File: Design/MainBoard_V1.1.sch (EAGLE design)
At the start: 65 parts, among them IC3 LM2936MP-3.3, Q1 25meg, Q4 2N3704, U1 STM32F20XR

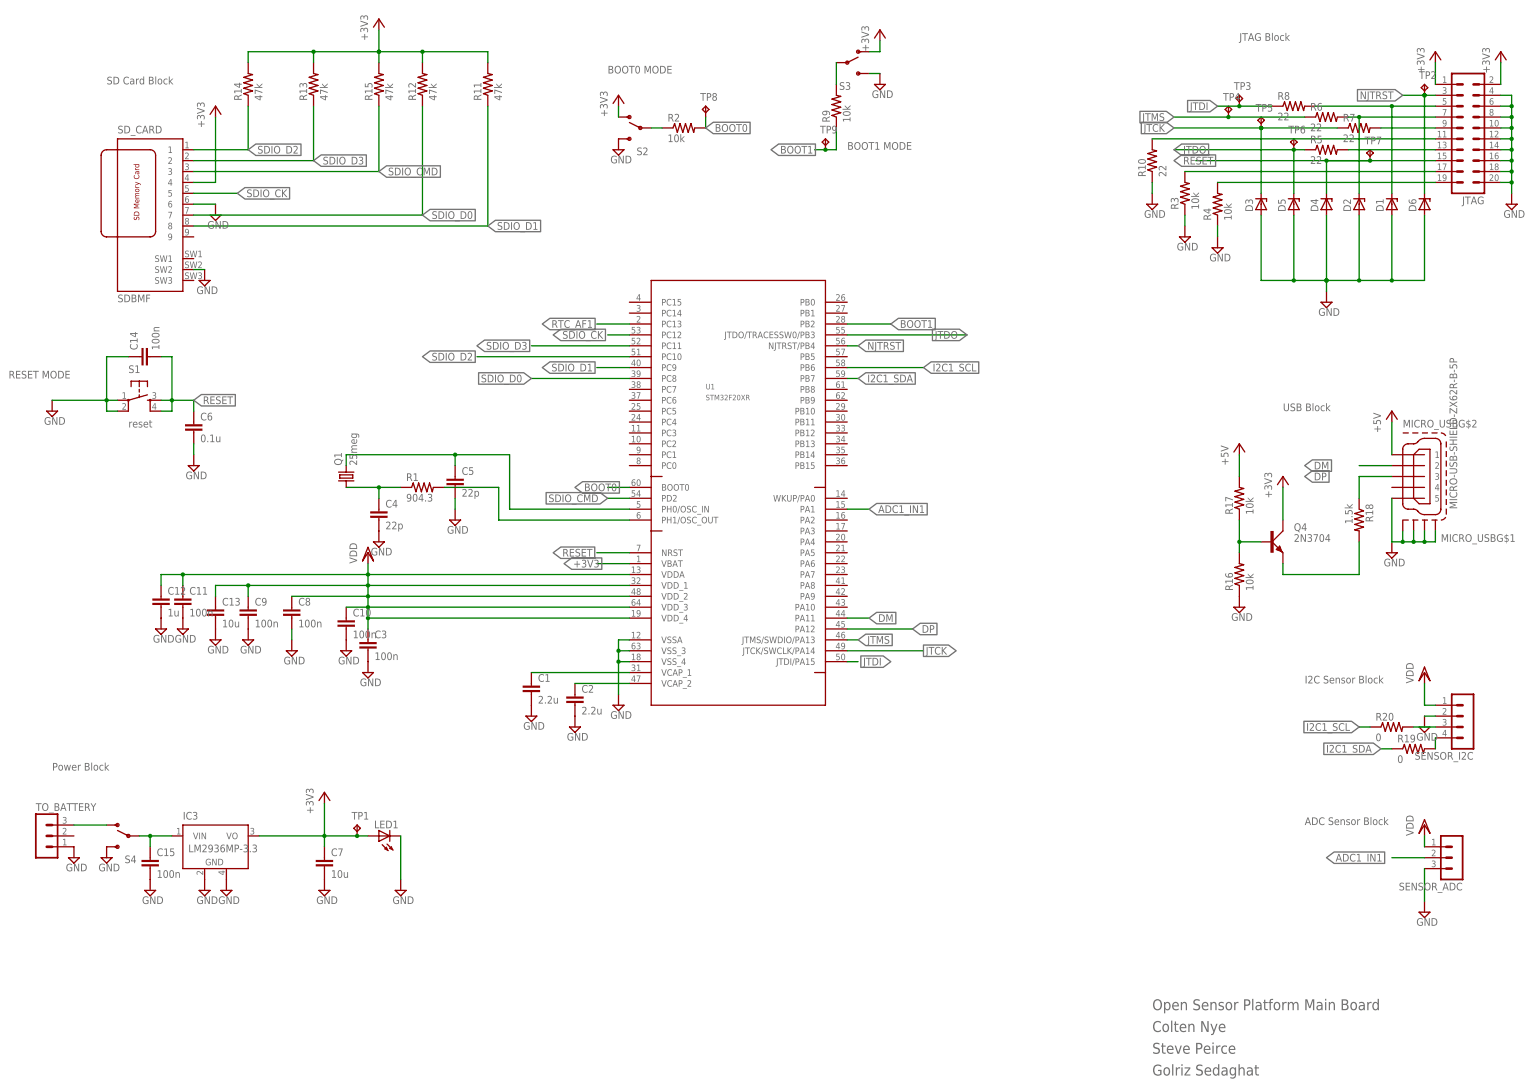
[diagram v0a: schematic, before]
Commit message: Document Revision
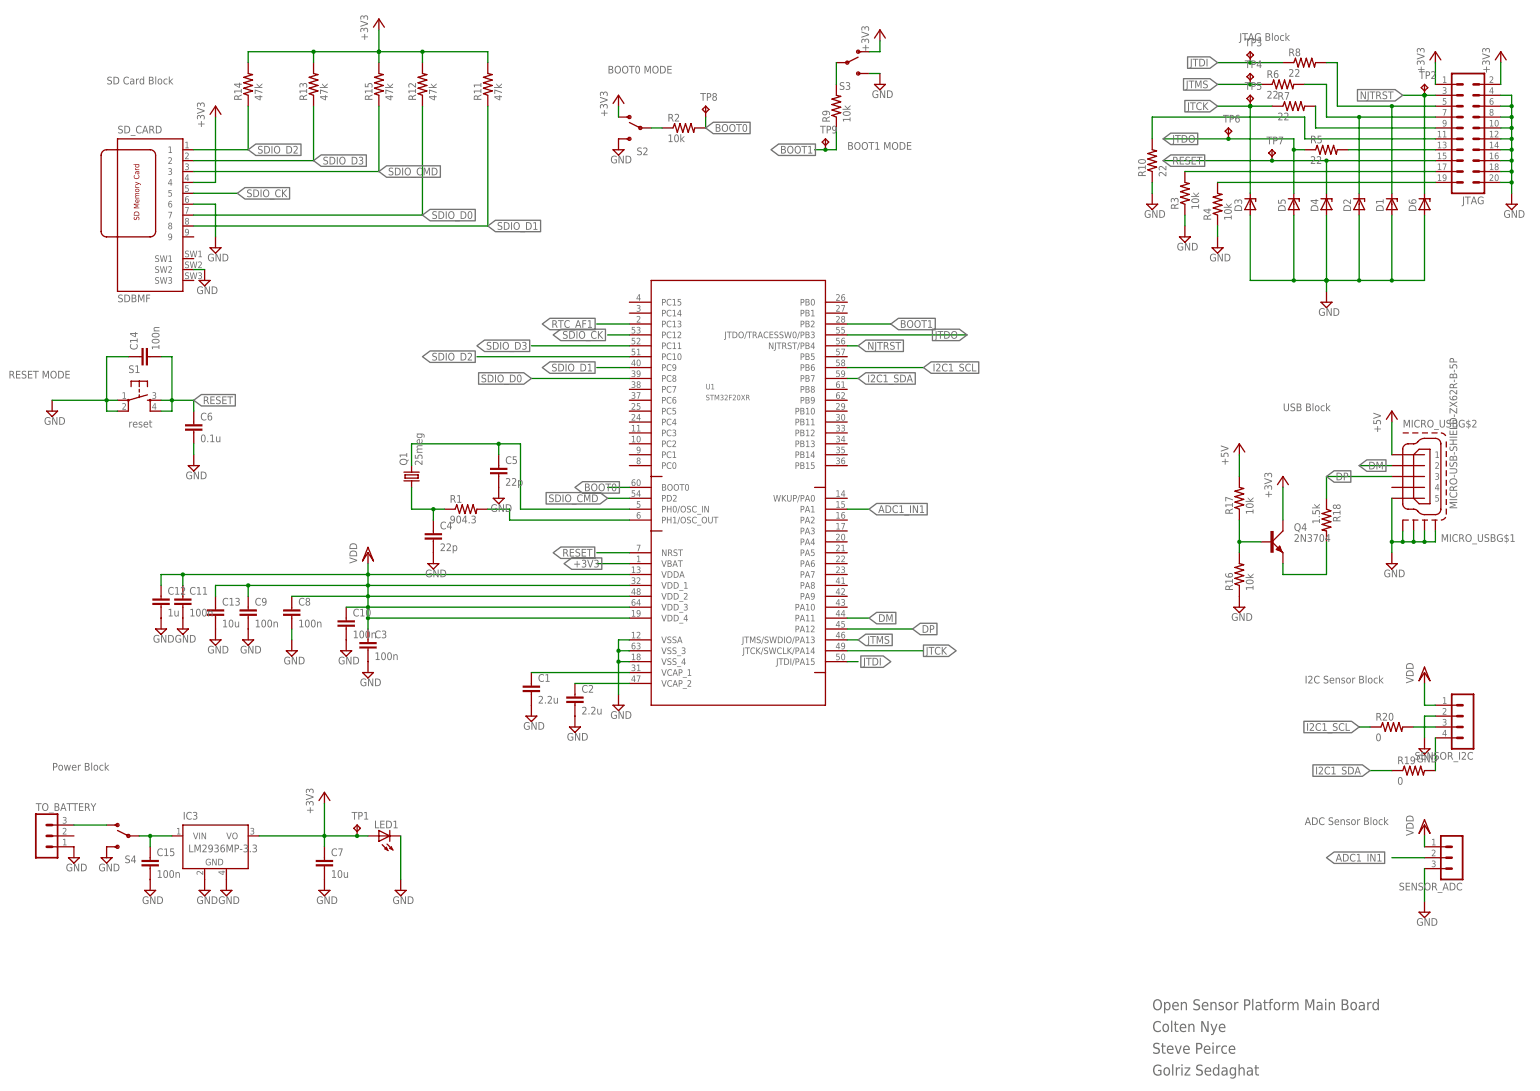
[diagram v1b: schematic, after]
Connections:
- net OSC_OUT renamed N$9
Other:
- moved on the sheet: C4, C5, D3, Q1, R1, R18, R19, R6, R7, R8, TP3, TP4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

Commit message: Revert "Document Revision"
This reverts commit 87a539b43a6471277175cce403c1623fabaade23.
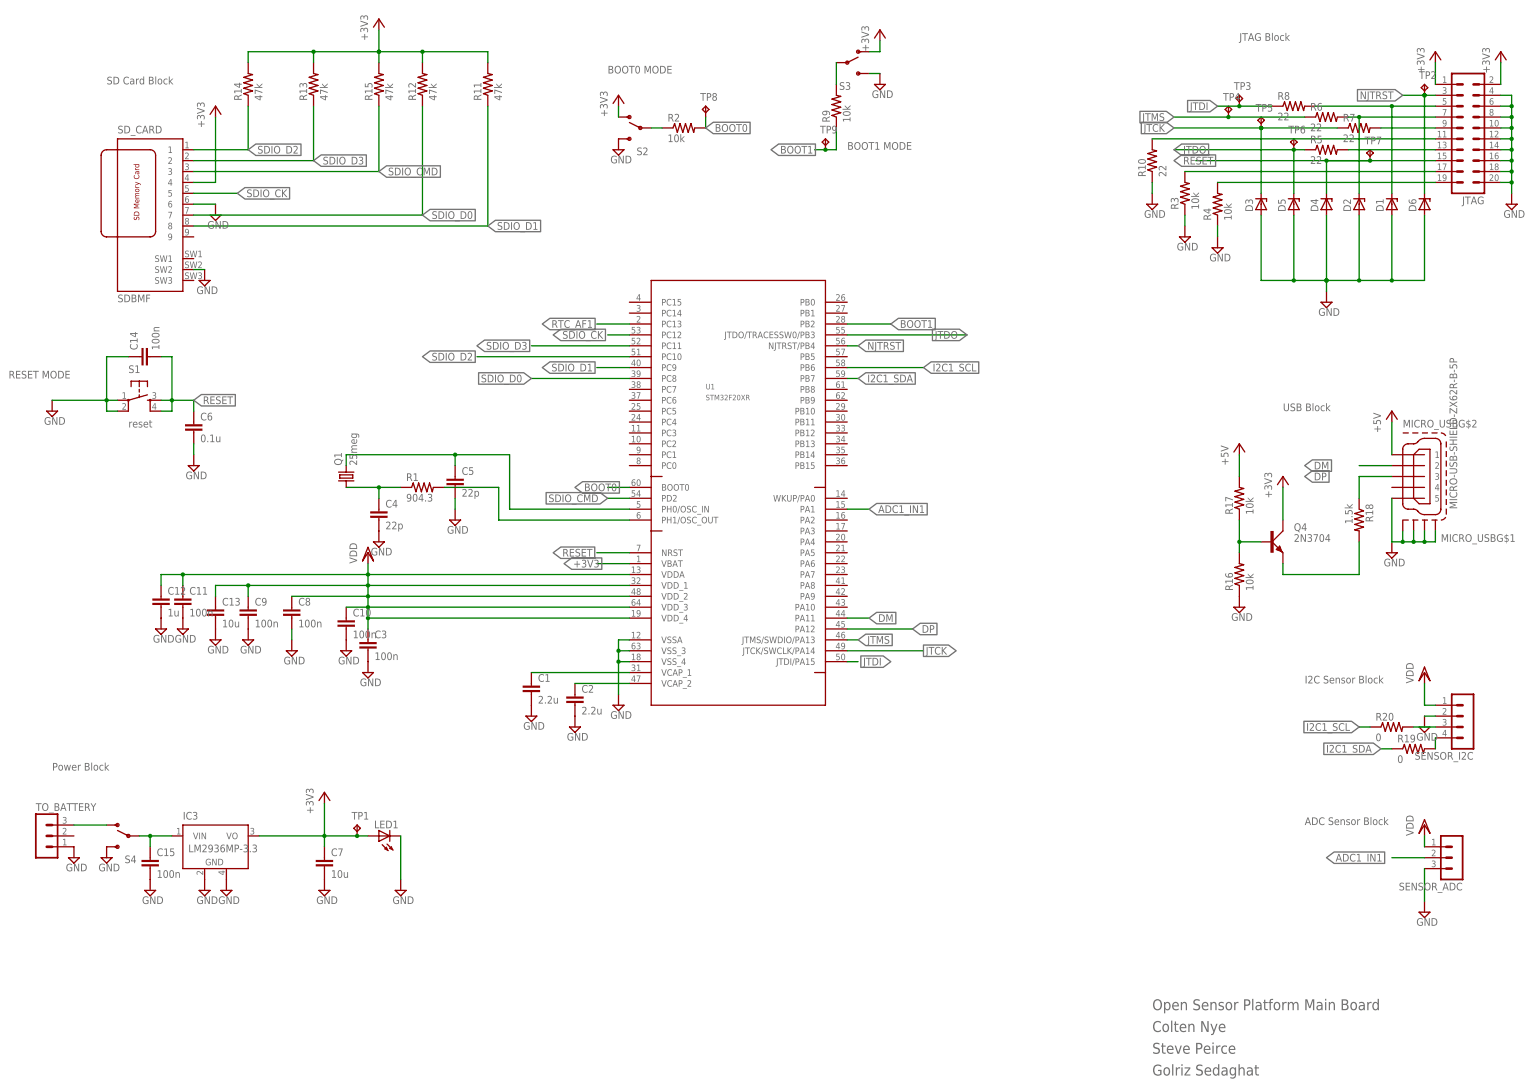
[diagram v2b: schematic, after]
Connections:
- net N$9 renamed OSC_OUT
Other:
- moved on the sheet: C4, C5, D3, Q1, R1, R18, R19, R6, R7, R8, TP3, TP4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
